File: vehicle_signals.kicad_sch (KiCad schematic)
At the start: 33 parts, among them IC4 TLIN1027DRQ1, U10 G3VM-61VY2, U11 G3VM-61VY2, U12 G3VM-61VY2, U13 G3VM-61VY2, U14 G3VM-61VY2, U15 G3VM-61VY2, U16 G3VM-61VY2, U17 G3VM-61VY2

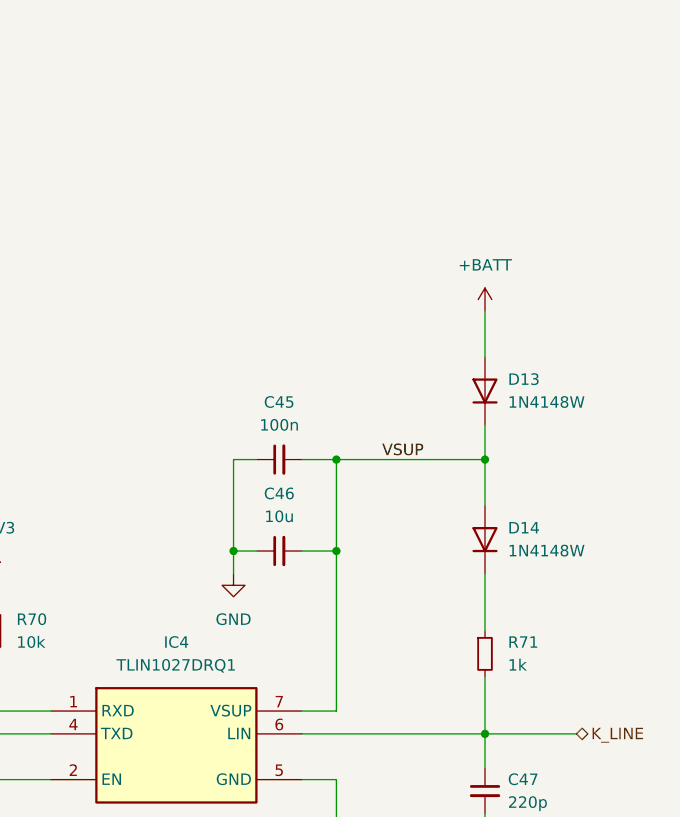
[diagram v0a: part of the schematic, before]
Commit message: brd: routing in progress
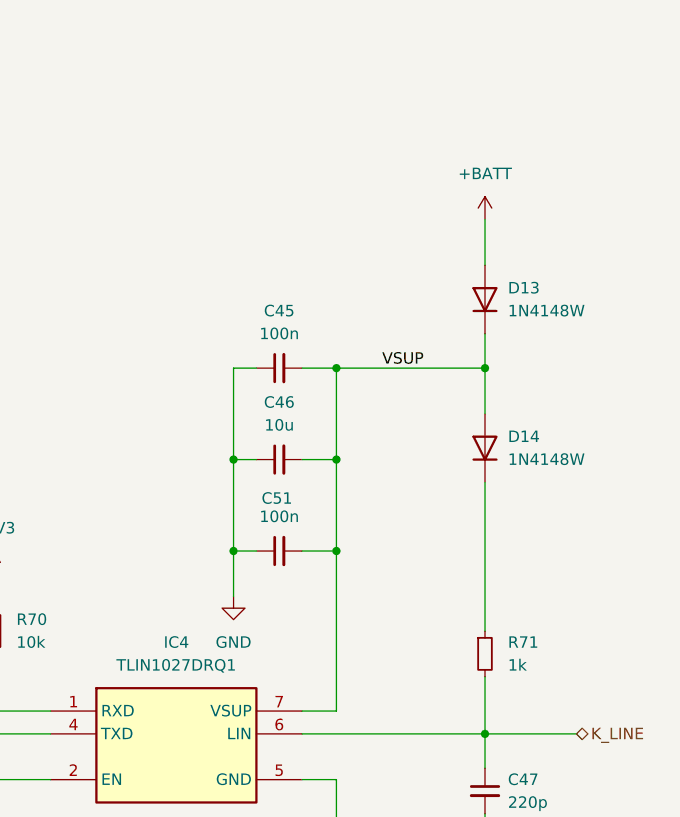
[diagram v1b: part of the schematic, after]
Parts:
- added C51: 100n, Capacitor_SMD:C_0603_1608Metric_Pad1.08x0.95mm_HandSolder, symbol Device:C_Small
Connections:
- net GND: now also C51.1
- net VSUP: now also C51.2
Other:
- moved on the sheet: C45, C46, D13, D14
